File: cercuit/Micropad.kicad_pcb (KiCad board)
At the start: 2 copper layers, 24 parts, among them SW1 SW_Push, SW10 SW_Push, SW11 SW_Push, SW12 SW_Push, SW2 SW_Push, SW3 SW_Push, SW4 SW_Push, SW5 SW_Push, SW6 SW_Push, SW7 SW_Push, SW8 SW_Push, SW9 SW_Push

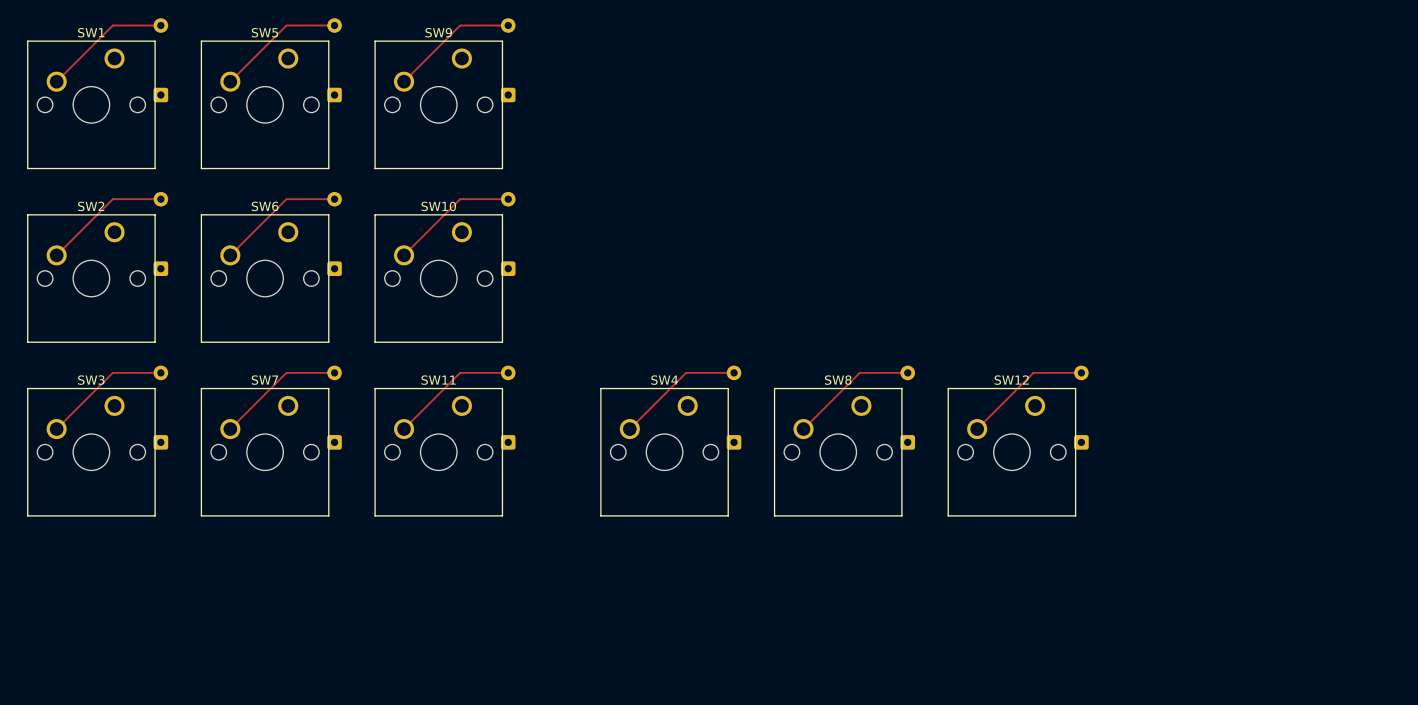
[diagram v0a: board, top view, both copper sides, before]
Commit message: pcb wiring
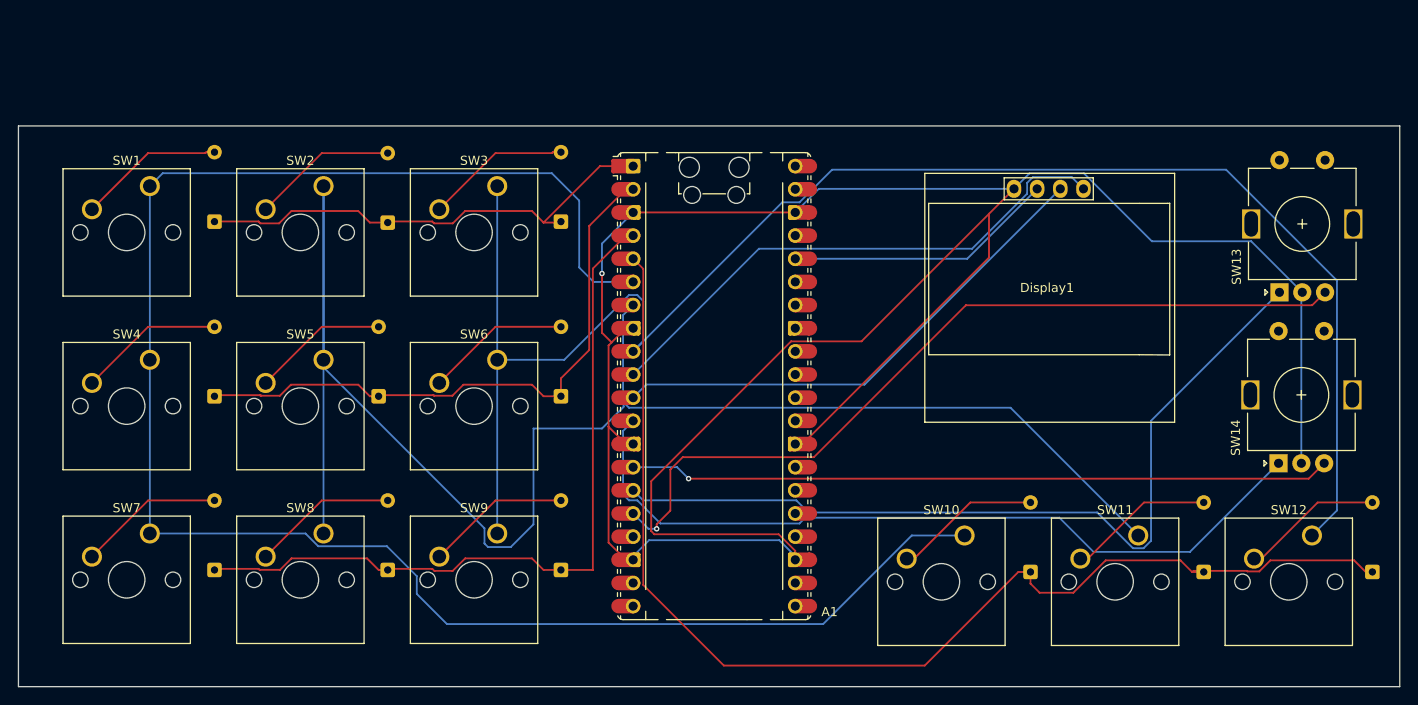
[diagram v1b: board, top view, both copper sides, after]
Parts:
- added A1: RaspberryPi_Pico, Module:RaspberryPi_Pico_Common_Unspecified, F.Cu at (144.3, 83.8)
- added Display1: Conn_01x07_Pin, Connector_Video:128x64OLED, F.Cu at (180.8, 72.8)
- added SW13: RotaryEncoder, Rotary_Encoder:RotaryEncoder_Alps_EC11E-Switch_Vertical_H20mm, F.Cu at (206.3, 73.6)
- added SW14: RotaryEncoder, Rotary_Encoder:RotaryEncoder_Alps_EC11E-Switch_Vertical_H20mm, F.Cu at (206.2, 92.3)
- moved SW11 75.5 mm to (190.8, 100.2)
- moved SW10 64.4 mm to (171.8, 100.2)
- moved SW8 60.6 mm to (101.5, 100.0)
- moved SW4 59.2 mm to (82.4, 81.0)
- moved SW9 52.2 mm to (120.5, 100.0)
- moved SW3 48.4 mm to (120.5, 61.9)
- moved D10 35.5 mm to (179.0, 104.2)
- moved D11 35.4 mm to (198.0, 104.2)
- moved D12 34.9 mm to (216.5, 104.2)
- moved SW12 33.5 mm to (209.9, 100.2)
- moved SW5 33.3 mm to (101.5, 81.0)
- moved SW6 26.9 mm to (120.5, 81.0)
- moved SW2 23.5 mm to (101.5, 61.9)
- moved SW7 20.6 mm to (82.4, 100.0)
- moved D4 15.2 mm to (89.5, 85.0)
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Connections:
- D10 pad 1: /Row 1 -> /Row 3
- D11 pad 1: /Row 2 -> /Row 3
- D2 pad 1: /Row 1 -> /Row 0
- D3 pad 1: /Row 2 -> /Row 0
- D4 pad 1: /Row 3 -> /Row 1
- D5 pad 1: /Row 0 -> /Row 1
- D8 pad 1: /Row 3 -> /Row 2
- D9 pad 1: /Row 0 -> /Row 2
- SW10 pad 1: /col 1 -> /col 0
- SW10 pad 2: Net-(D6-A) -> Net-(D10-A)
- SW11 pad 1: /col 2 -> /col 1
- SW11 pad 2: Net-(D9-A) -> Net-(D11-A)
- SW2 pad 1: /col 0 -> /col 1
- SW2 pad 2: Net-(D4-A) -> Net-(D2-A)
- SW3 pad 1: /col 1 -> /col 2
- SW3 pad 2: Net-(D7-A) -> Net-(D3-A)
- SW4 pad 1: /col 2 -> /col 0
- SW4 pad 2: Net-(D10-A) -> Net-(D4-A)
- SW5 pad 1: /col 0 -> /col 1
- SW5 pad 2: Net-(D2-A) -> Net-(D5-A)
- SW6 pad 1: /col 1 -> /col 2
- SW6 pad 2: Net-(D5-A) -> Net-(D6-A)
- SW7 pad 1: /col 1 -> /col 0
- SW7 pad 2: Net-(D8-A) -> Net-(D7-A)
- SW8 pad 1: /col 2 -> /col 1
- SW8 pad 2: Net-(D11-A) -> Net-(D8-A)
- SW9 pad 1: /col 0 -> /col 2
- SW9 pad 2: Net-(D3-A) -> Net-(D9-A)
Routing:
- net GND: track 0.00 -> 278.3 mm, vias 0 -> 1
- net /col 0: track 0.00 -> 199.6 mm
- net /col 1: track 0.00 -> 186.7 mm
- net /col 2: track 0.00 -> 182.9 mm
- net /Row 3: track 0.00 -> 129.3 mm
- net Net-(A1-GPIO11): track 0.00 -> 92.9 mm
- net Net-(A1-GPIO12): track 0.00 -> 90.3 mm, vias 0 -> 1
- net Net-(A1-GPIO9): track 0.00 -> 87.6 mm
- net /Row 2: track 0.00 -> 82.0 mm
- net Net-(A1-GPIO10): track 0.00 -> 77.0 mm, vias 0 -> 1
- net /Row 1: track 0.00 -> 65.9 mm
- net /SDA: track 0.00 -> 59.6 mm
- net /SCK: track 0.00 -> 56.3 mm
- net /Row 0: track 0.00 -> 52.0 mm
- net +3.3V: track 0.00 -> 29.7 mm
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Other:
- board outline added: 151.5 x 61.5 mm
